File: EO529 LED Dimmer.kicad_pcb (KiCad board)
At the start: 2 copper layers, 50.8 x 59.7 mm, 35 parts, among them J1 VBat, Q1 BC639, Q2 BC639, Q3 BC639, Q4 BC639, U1 LM339, U2 NE555P

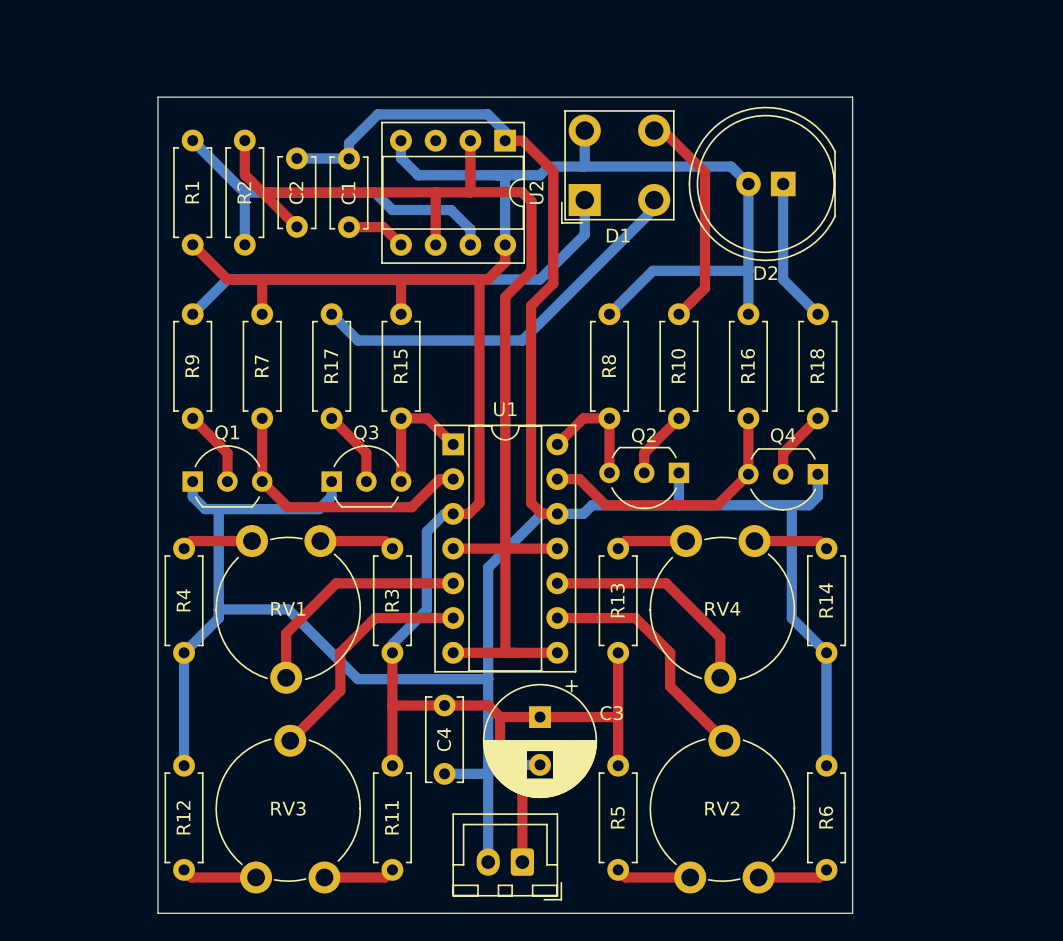
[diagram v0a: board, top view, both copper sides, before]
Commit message: Revert "New layout, less parts"
This reverts commit 43836197f3911cfe2976812753205c060315a555.
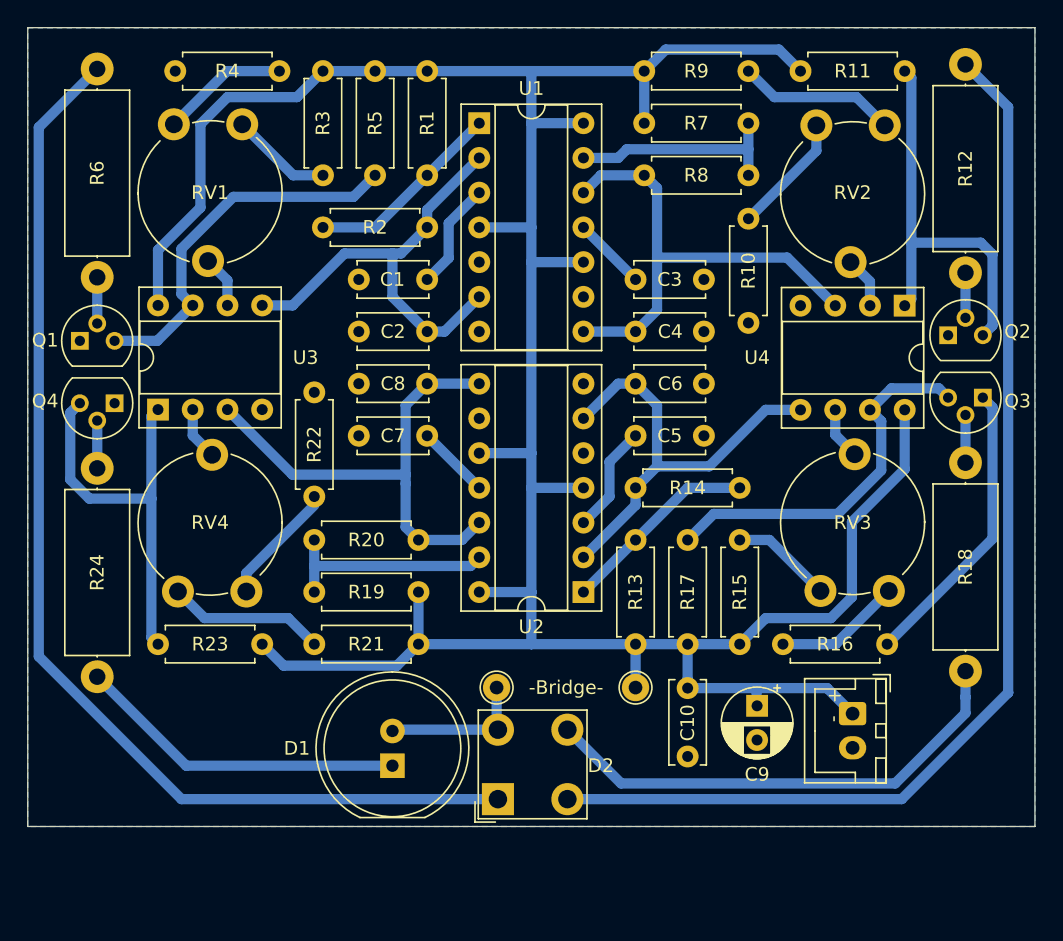
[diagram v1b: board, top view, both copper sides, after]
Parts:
- added C10: 100n, Capacitor_THT:C_Disc_D6.0mm_W2.5mm_P5.00mm, F.Cu at (114.9, 117.6)
- added C5: 10n, Capacitor_THT:C_Disc_D5.0mm_W2.5mm_P5.00mm, F.Cu at (111.1, 99.1)
- added C6: 10n, Capacitor_THT:C_Disc_D5.0mm_W2.5mm_P5.00mm, F.Cu at (111.1, 95.3)
- added C7: 10n, Capacitor_THT:C_Disc_D5.0mm_W2.5mm_P5.00mm, F.Cu at (95.9, 99.1)
- added C8: 10n, Capacitor_THT:C_Disc_D5.0mm_W2.5mm_P5.00mm, F.Cu at (95.9, 95.3)
- added C9: 10u, Capacitor_THT:CP_Radial_D5.0mm_P2.50mm, F.Cu at (120.0, 118.9)
- added R19: 10k, Resistor_THT:R_Axial_DIN0207_L6.3mm_D2.5mm_P7.62mm_Horizontal, F.Cu at (95.2, 110.6)
- added R20: 10k, Resistor_THT:R_Axial_DIN0207_L6.3mm_D2.5mm_P7.62mm_Horizontal, F.Cu at (87.6, 106.7)
- added R21: 82k, Resistor_THT:R_Axial_DIN0207_L6.3mm_D2.5mm_P7.62mm_Horizontal, F.Cu at (95.2, 114.4)
- added R22: 82k, Resistor_THT:R_Axial_DIN0207_L6.3mm_D2.5mm_P7.62mm_Horizontal, F.Cu at (87.6, 103.6)
- added R23: 4.7k, Resistor_THT:R_Axial_DIN0207_L6.3mm_D2.5mm_P7.62mm_Horizontal, F.Cu at (76.2, 114.4)
- added R24: 220, Resistor_THT:R_Axial_DIN0414_L11.9mm_D4.5mm_P15.24mm_Horizontal, F.Cu at (71.8, 101.5)
- added TP1: TestPoint, TestPoint:TestPoint_THTPad_D2.0mm_Drill1.0mm, F.Cu at (101.0, 117.5)
- added TP2: TestPoint, TestPoint:TestPoint_THTPad_D2.0mm_Drill1.0mm, F.Cu at (111.1, 117.5)
- added U3: LM393, Package_DIP:DIP-8_W7.62mm_Socket, F.Cu at (76.2, 97.2)
- added U4: LM393, Package_DIP:DIP-8_W7.62mm_Socket, F.Cu at (130.8, 89.6)
- C3: value 100u -> 10n; footprint Capacitor_THT:CP_Radial_D8.0mm_P3.50mm -> Capacitor_THT:C_Disc_D5.0mm_W2.5mm_P5.00mm
- C4: value 100n -> 10n; footprint Capacitor_THT:C_Disc_D6.0mm_W2.5mm_P5.00mm -> Capacitor_THT:C_Disc_D5.0mm_W2.5mm_P5.00mm
- D1: value LED_RGBA -> White; footprint LED_THT:LED_BL-FL7680RGB -> LED_THT:LED_D10.0mm
- D2: value White -> LED_RGBA; footprint LED_THT:LED_D10.0mm -> LED_THT:LED_BL-FL7680RGB
- Q1, Q2, Q3, Q4: footprint Package_TO_SOT_THT:TO-92_Inline_Wide -> Package_TO_SOT_THT:TO-92
- R10: value 180 -> 82k
- R11, R5: value 82k -> 4.7k
- R12: value 82k -> 180; footprint Resistor_THT:R_Axial_DIN0207_L6.3mm_D2.5mm_P7.62mm_Horizontal -> Resistor_THT:R_Axial_DIN0414_L11.9mm_D4.5mm_P15.24mm_Horizontal
- R13, R14: value 82k -> 10k
- R15, R16: value 4.7k -> 82k
- R17: value 180 -> 4.7k
- R18: value 220 -> 180; footprint Resistor_THT:R_Axial_DIN0207_L6.3mm_D2.5mm_P7.62mm_Horizontal -> Resistor_THT:R_Axial_DIN0414_L11.9mm_D4.5mm_P15.24mm_Horizontal
- R6: value 82k -> 150; footprint Resistor_THT:R_Axial_DIN0207_L6.3mm_D2.5mm_P7.62mm_Horizontal -> Resistor_THT:R_Axial_DIN0414_L11.9mm_D4.5mm_P15.24mm_Horizontal
- R7, R8: value 4.7k -> 10k
- R9: value 150 -> 82k
- U1: value LM339 -> NE556
- U2: value NE555P -> NE556; footprint Package_DIP:DIP-8_W7.62mm_Socket -> Package_DIP:DIP-14_W7.62mm_Socket
- moved R12 71.9 mm to (135.3, 87.2)
- moved R6 68.7 mm to (71.8, 87.5)
- moved R11 63.1 mm to (130.8, 72.5), turned to 180 degrees
- moved RV2 55.2 mm to (124.3, 76.4), turned to -90 degrees
- moved Q4 51.7 mm to (73.0, 96.7)
- moved D2 49.6 mm to (101.1, 125.7), turned to 90 degrees
- moved Q3 48.0 mm to (136.5, 96.3), turned to 180 degrees
- moved R5 46.7 mm to (92.1, 80.1), turned to 90 degrees
- moved RV3 46.3 mm to (129.6, 110.5)
- moved D1 43.7 mm to (93.3, 123.3)
- moved R3 42.8 mm to (88.3, 72.5), turned to -90 degrees
- moved R9 41.7 mm to (111.8, 72.5), turned to 0 degrees
- moved R4 35.6 mm to (85.1, 72.5), turned to 180 degrees
- moved R7 35.3 mm to (111.8, 76.3), turned to 0 degrees
- moved U2 33.5 mm to (107.3, 110.6), turned to 180 degrees
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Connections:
- C2 pad 1: PWM -> Net-(C2-Pad1)
- C3 pad 1: VCC -> Net-(C3-Pad1)
- C4 pad 1: VCC -> Net-(C4-Pad1)
- D1 pad 1: Red -> Net-(D1-Pad1)
- D1 pad 2: Green -> V_LED
- D2 pad 1: Net-(D2-Pad1) -> Red
- D2 pad 2: VCC -> Green
- R10 pad 1: Net-(Q2-Pad2) -> Net-(R10-Pad1)
- R10 pad 2: Blue -> GND
- R11 pad 1: VCC -> Net-(Q2-Pad3)
- R11 pad 2: Net-(R11-Pad2) -> VCC
- R12 pad 1: Net-(R12-Pad1) -> Net-(Q2-Pad2)
- R12 pad 2: GND -> Green
- R14 pad 1: Net-(R14-Pad1) -> Net-(R13-Pad2)
- R14 pad 2: GND -> Net-(C6-Pad1)
- R15 pad 1: Net-(Q3-Pad3) -> VCC
- R15 pad 2: VCC -> Net-(R15-Pad2)
- R16 pad 1: Net-(Q4-Pad3) -> Net-(R16-Pad1)
- R16 pad 2: VCC -> GND
- R17 pad 1: Net-(Q3-Pad2) -> Net-(Q3-Pad3)
- R17 pad 2: Green -> VCC
- R18 pad 1: Net-(Q4-Pad2) -> Net-(Q3-Pad2)
- R18 pad 2: Net-(D2-Pad1) -> Blue
- R2 pad 2: PWM -> Net-(C2-Pad1)
- R5 pad 1: VCC -> Net-(Q1-Pad3)
- R5 pad 2: Net-(R5-Pad2) -> VCC
- R6 pad 1: Net-(R6-Pad1) -> Net-(Q1-Pad2)
- R6 pad 2: GND -> Red
- R7 pad 1: Net-(Q1-Pad3) -> VCC
- R7 pad 2: VCC -> Net-(R7-Pad2)
- R8 pad 1: Net-(Q2-Pad3) -> Net-(R7-Pad2)
- R8 pad 2: VCC -> Net-(C4-Pad1)
- R9 pad 1: Net-(Q1-Pad2) -> VCC
- R9 pad 2: Red -> Net-(R9-Pad2)
- RV2 pad 1: Net-(R6-Pad1) -> Net-(R10-Pad1)
- RV2 pad 3: Net-(R5-Pad2) -> Net-(R9-Pad2)
- RV3 pad 1: Net-(R11-Pad2) -> Net-(R16-Pad1)
- RV3 pad 2: Net-(U1-Pad6) -> Net-(RV3-Pad2)
- RV3 pad 3: Net-(R12-Pad1) -> Net-(R15-Pad2)
- RV4 pad 1: Net-(R13-Pad2) -> Net-(R22-Pad1)
- RV4 pad 3: Net-(R14-Pad1) -> Net-(R21-Pad2)
- U1 pad 1: Net-(Q3-Pad3) -> Net-(R1-Pad2)
- U1 pad 10: Net-(RV4-Pad2) -> VCC
- U1 pad 11: PWM -> Net-(C3-Pad1)
- U1 pad 12: GND -> Net-(C4-Pad1)
- U1 pad 13: Net-(Q4-Pad3) -> Net-(R7-Pad2)
- U1 pad 14: Net-(Q2-Pad3) -> VCC
- U1 pad 2: Net-(Q1-Pad3) -> Net-(C2-Pad1)
- U1 pad 3: VCC -> Net-(C1-Pad1)
- U1 pad 4: PWM -> VCC
- U1 pad 5: Net-(RV1-Pad2) -> unconnected-(U1-Pad5)
- U1 pad 6: Net-(U1-Pad6) -> Net-(C2-Pad1)
- U1 pad 7: PWM -> GND
- U1 pad 8: PWM -> Net-(C4-Pad1)
- U1 pad 9: Net-(RV2-Pad2) -> unconnected-(U1-Pad9)
- U2 pad 1: GND -> Net-(R13-Pad2)
- U2 pad 2: PWM -> Net-(C6-Pad1)
- U2 pad 3: unconnected-(U2-Pad3) -> Net-(C5-Pad1)
- U2 pad 5: Net-(C1-Pad1) -> unconnected-(U2-Pad5)
- U2 pad 6: PWM -> Net-(C6-Pad1)
- U2 pad 7: Net-(R1-Pad2) -> GND
- U2 pad 8: VCC -> Net-(C8-Pad1)
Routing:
- net GND: track 183.7 -> 21.5 mm
- net PWM: track 84.7 -> 0.00 mm
- net Green: track 29.0 -> 82.7 mm
- net VCC: track 163.3 -> 215.4 mm
- net Red: track 33.6 -> 82.6 mm
- net Net-(C8-Pad1): track 0.00 -> 36.3 mm
- net Net-(C4-Pad1): track 0.00 -> 35.7 mm
- net Net-(C2-Pad1): track 0.00 -> 32.7 mm
- net Net-(C6-Pad1): track 0.00 -> 32.6 mm
- net Net-(D1-Pad1): track 0.00 -> 24.3 mm
- net Net-(Q2-Pad3): track 8.58 -> 30.1 mm
- net Blue: track 16.4 -> 35.9 mm
- net Net-(Q3-Pad3): track 9.22 -> 27.7 mm
- net Net-(U1-Pad6): track 17.3 -> 0.00 mm
- net Net-(R7-Pad2): track 0.00 -> 16.1 mm
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- added copper zone on B.Cu, net GND
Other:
- board size 50.8 x 59.7 mm -> 73.7 x 58.4 mm
- board text added: "- +"
- board text added: "-Bridge-"
